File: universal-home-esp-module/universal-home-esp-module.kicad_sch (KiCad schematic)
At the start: 8 parts, among them J1 ES8311 CODEC, J2 LDR MOD, J3 RELAYS, J4 RGB LED, J5 ENV SENSOR, J6 5V PWR, U1 ESP32-C3_SUPERMINI_SMD, U2 74HC595

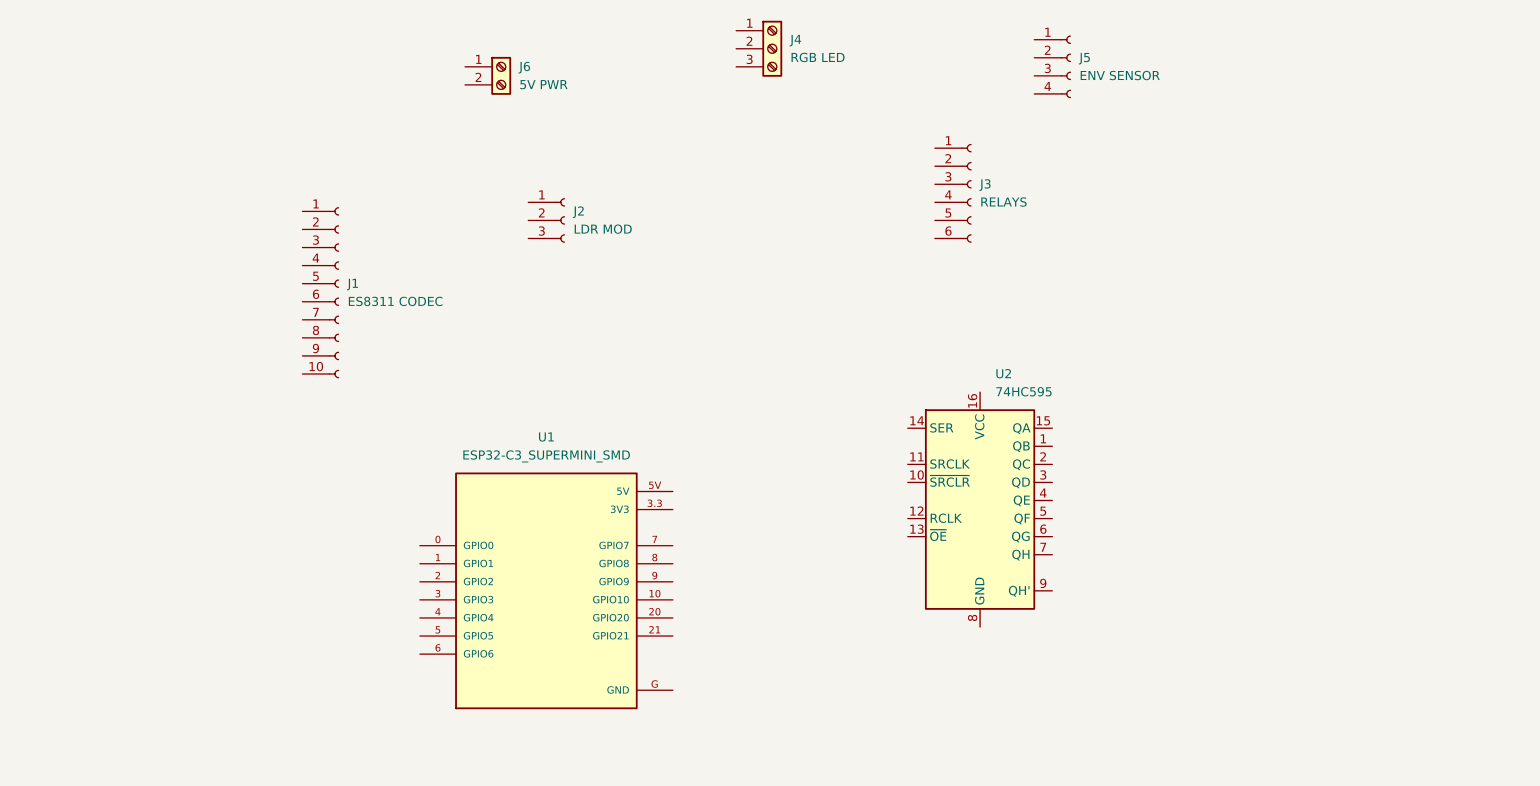
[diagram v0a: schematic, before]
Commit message: updated schematic
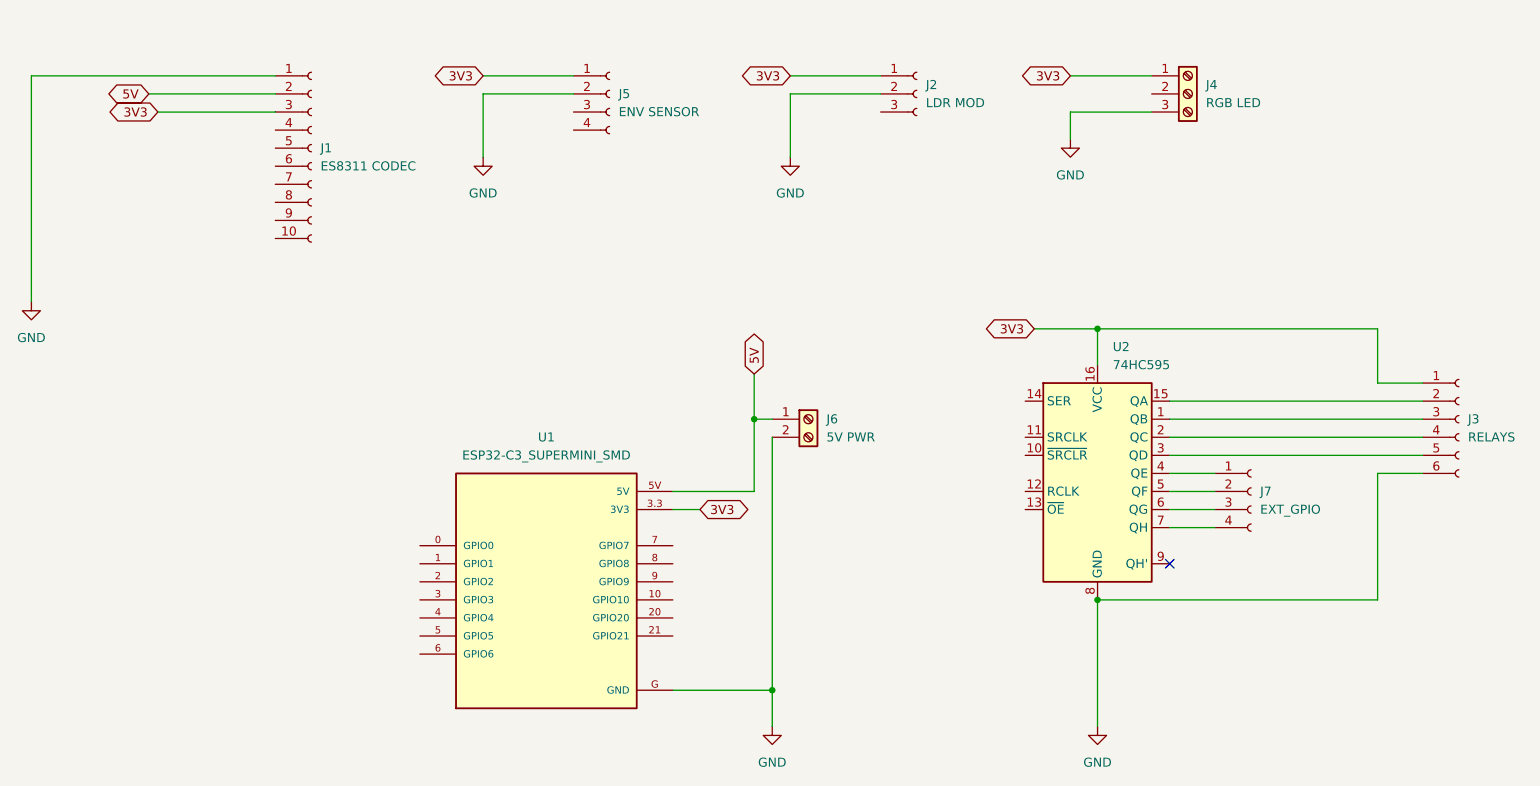
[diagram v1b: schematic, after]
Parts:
- added J7: EXT_GPIO, Connector_PinHeader_2.54mm:PinHeader_1x04_P2.54mm_Vertical, symbol Connector:Conn_01x04_Socket
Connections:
- net GND: now reaches J1.1 (Pin_1)
- net GND: now also J2.2 (Pin_2), J3.6 (Pin_6), J4.3 (Pin_3), J5.2 (Pin_2), J6.2 (Pin_2), U1.G (GND), U2.8 (GND)
- net 5V: now reaches J1.2 (Pin_2)
- net 5V: now also J6.1 (Pin_1), U1.5V
- net 3V3: now reaches J1.3 (Pin_3)
- net 3V3: now also J2.1 (Pin_1), J3.1 (Pin_1), J4.1 (Pin_1), J5.1 (Pin_1), U1.3.3 (3V3), U2.16 (VCC)
- net at U2.1 (QB): now also J3.3 (Pin_3)
- net at U2.15 (QA): now also J3.2 (Pin_2)
- net at U2.2 (QC): now also J3.4 (Pin_4)
- net at U2.3 (QD): now also J3.5 (Pin_5)
- net at U2.4 (QE): now also J7.1 (Pin_1)
- net at U2.5 (QF): now also J7.2 (Pin_2)
- net at U2.6 (QG): now also J7.3 (Pin_3)
- net at U2.7 (QH): now also J7.4 (Pin_4)
- no-connect marks 0 -> 1
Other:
- moved on the sheet: J1, J2, J3, J4, J5, J6, U2
